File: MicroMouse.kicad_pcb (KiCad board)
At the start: 2 copper layers, 100 x 80 mm, 78 parts, among them CN11 mouseBattery, Q1 IRLML6402, Q2 IRLML6344, SW1 SPST, SW2 SPST, SW3 SPST, U1 FULL_LED_A, U2 STM32F405RGTx, U3 TB6612, U4 CN_MOTOR, U5 CN_MOTOR, U6 MPU9250, U7 ZH

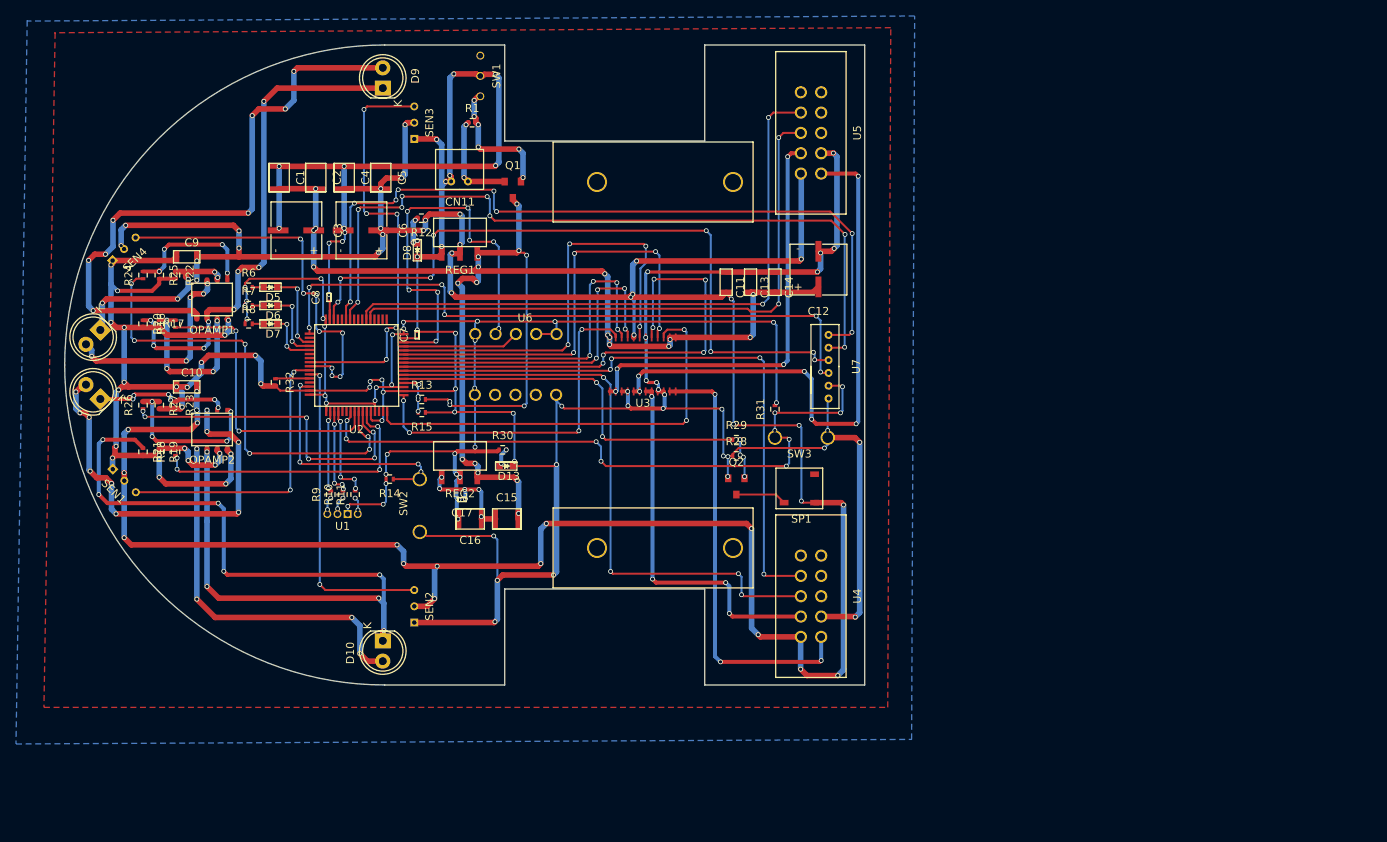
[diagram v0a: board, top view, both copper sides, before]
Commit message: 修正後
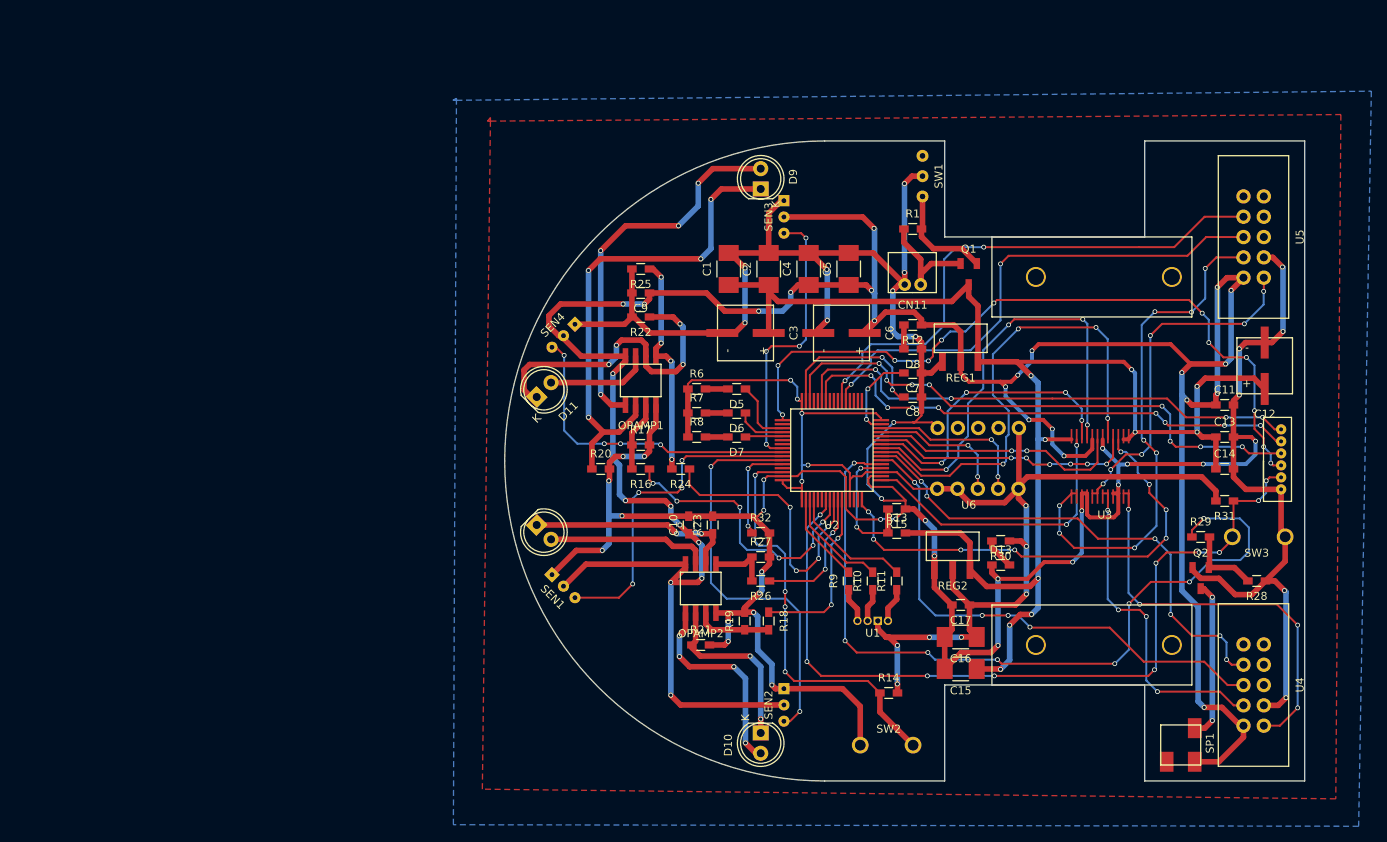
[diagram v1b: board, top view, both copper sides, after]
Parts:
- removed the REF** at (6.05, 0.13)
- removed the REF** at (6.05, 45.9)
- added REF**: motormount, myfootprint:motormount, F.Cu at (60.9, 12.0)
- added REF**: motormount, myfootprint:motormount, F.Cu at (60.9, 58.0)
- C1, C15, C16, C2, C4, C5: footprint myfootprint:GRM32EB31C476KE15 -> Resistors_SMD:R_1210_HandSoldering
- C10, C11, C13, C14, C9: footprint myfootprint:CL31A106KBHNNNE -> Resistors_SMD:R_0603_HandSoldering
- C17, C7, C8: footprint myfootprint:C1005X7R1H104K050BB -> Resistors_SMD:R_0603_HandSoldering
- D13, D5, D6, D7, D8: footprint myfootprint:OSTG1608C1A -> Resistors_SMD:R_0603_HandSoldering
- R1, R10, R11, R12, R13, R14, R15, R16, R17, R18, R19, R20, R21, R22, R23, R24, R25, R26, R27, R28, R29, R30, R31, R32, R6, R7, R8, R9: footprint Resistors_SMD:R_0402 -> Resistors_SMD:R_0603_HandSoldering
- moved R26 80.3 mm to (32.0, 55.0), turned to 180 degrees
- moved R27 77.5 mm to (32.0, 52.0), turned to 0 degrees
- moved R18 77.1 mm to (33.0, 60.0), turned to 270 degrees
- moved R19 76.2 mm to (30.0, 60.0), turned to 90 degrees
- moved C8 75.2 mm to (51.0, 32.0), turned to 180 degrees
- moved R21 73.8 mm to (24.5, 63.0), turned to 0 degrees
- moved R24 71.4 mm to (22.0, 41.0), turned to 180 degrees
- moved R23 68.8 mm to (26.0, 48.0), turned to 90 degrees
- moved R11 68.6 mm to (49.0, 55.0)
- moved R14 67.9 mm to (48.0, 69.0), turned to 0 degrees
- moved U1 67.6 mm to (46.0, 61.0)
- moved R10 67.1 mm to (46.0, 55.0)
- moved R28 66.9 mm to (94.0, 55.0), turned to 180 degrees
- moved SW2 66.6 mm to (48.0, 74.0), turned to 180 degrees
- moved R9 65.6 mm to (43.0, 55.0)
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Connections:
- C15 pad 2: Net-(C15-Pad2) -> GND
- C16 pad 2: Net-(C15-Pad2) -> GND
- C17 pad 2: Net-(C15-Pad2) -> GND
- REG2 pad 1: Net-(C15-Pad2) -> GND
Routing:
- net Net-(D10-Pad1): track 105.1 -> 22.4 mm, vias 9 -> 2
- net SPK: track 47.8 -> 99.0 mm, vias 2 -> 8
- net +5V: track 381.1 -> 342.1 mm, vias 48 -> 28
- net GND: track 502.1 -> 466.1 mm, vias 78 -> 42
- net USART1_RX: track 97.4 -> 65.1 mm, vias 8 -> 4
- net USART1_TX: track 95.8 -> 64.1 mm
- net Net-(D12-Pad2): track 51.3 -> 20.4 mm, vias 10 -> 0
- net Net-(D9-Pad2): track 77.9 -> 47.5 mm, vias 8 -> 4
- net SDA: track 50.8 -> 20.9 mm, vias 8 -> 2
- net Net-(U3-Pad5): track 71.7 -> 43.4 mm
- net LED_LF: track 41.6 -> 17.0 mm, vias 6 -> 2
- net M_STBY: track 54.9 -> 32.0 mm, vias 4 -> 2
- net M_IN2_R: track 55.0 -> 32.9 mm, vias 4 -> 6
- net LED_RF: track 57.6 -> 35.6 mm, vias 6 -> 4
- net Net-(D10-Pad2): track 47.3 -> 25.7 mm
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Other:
- rule via_min_size: 0.6 -> 0.4
